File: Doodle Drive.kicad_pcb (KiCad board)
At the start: 2 copper layers, 62.9 x 80 mm, 101 parts, among them J1 USB_B, J12 PINHD_1x4_Male, J15 PINHD_1x4_Male, J2 PINHD_1x4_Male, J3 Screw_Terminal_01x02, J6 PINHD_1x2_Male, J8 PINHD_1x4_Male, J9 PINHD_1x4_Male, SW1 Push_Button, SW2 Push_Button, SW3 Push_Button, U1 STM32F411RETx, U2 DRV8825PWP, U3 DRV8825PWP, U4 DRV8825PWP, U5 DRV8825PWP, U6 AP7343-30W5-7, U7 CP2102-GMR_NRND, Y1 32.768KHz ±20ppm 12.5pF, Y2 25MHZ 9PF

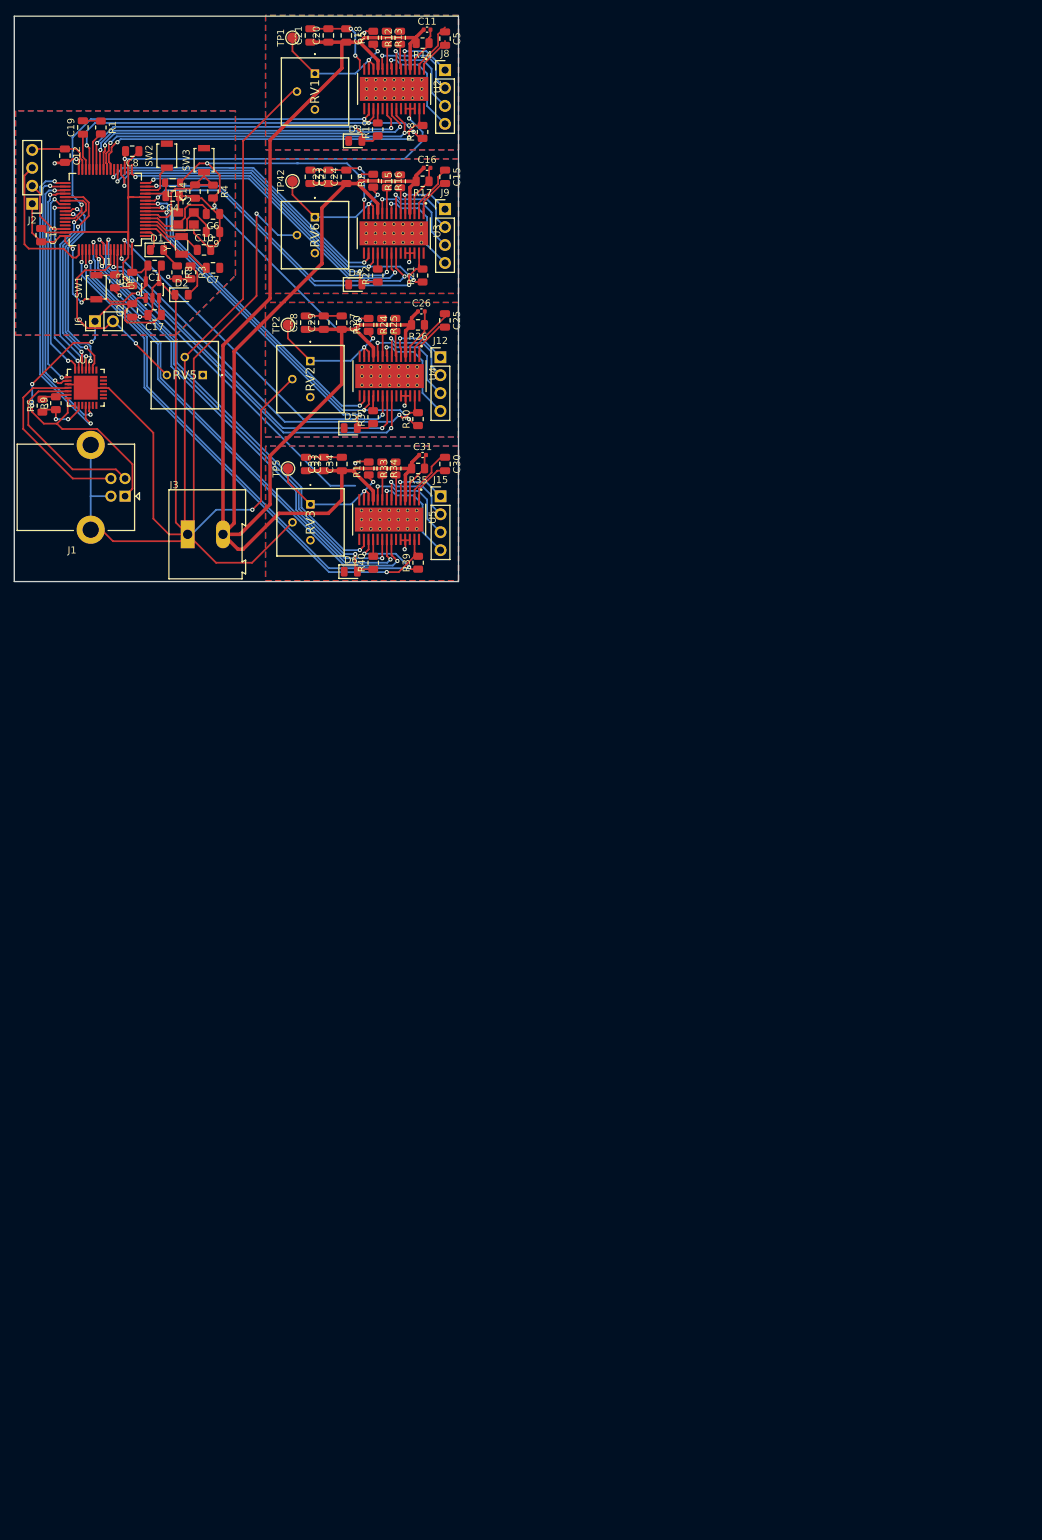
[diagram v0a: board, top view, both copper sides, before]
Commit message: deTommaso approved version
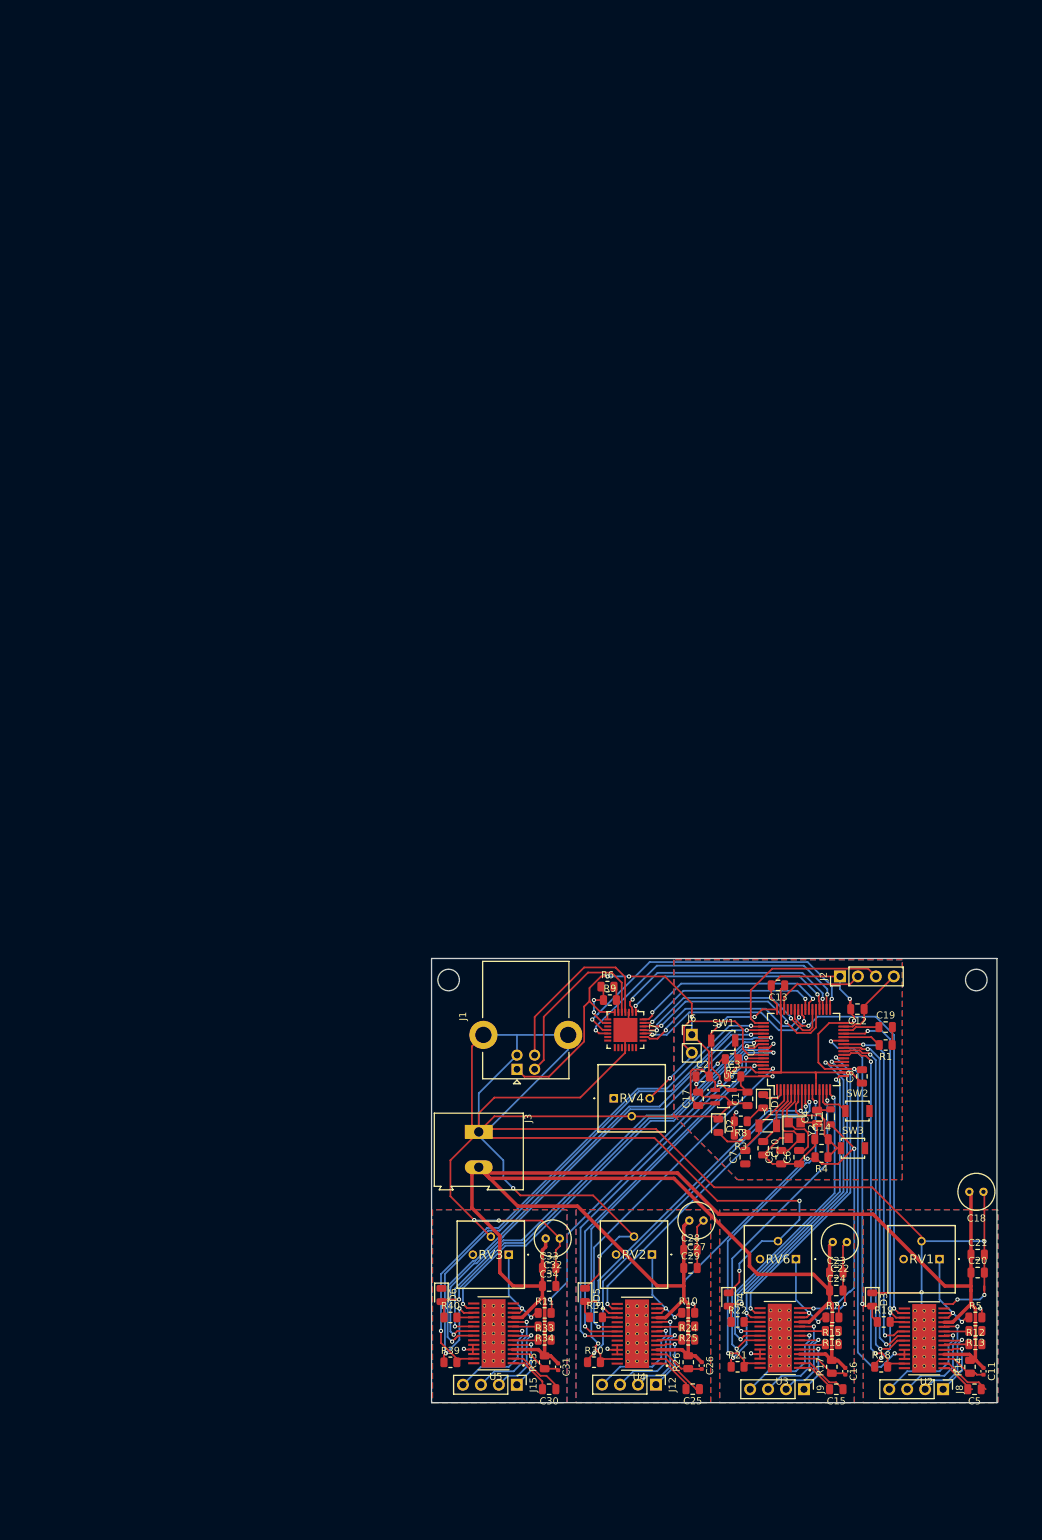
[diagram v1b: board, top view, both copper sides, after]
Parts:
- removed RV5: R_Potentiometer, poti:3386P1473LF
- removed TP1, TP2, TP42, TP5: TestPoint, TestPoint:TestPoint_Pad_D1.5mm
- added RV4: R_Potentiometer, poti:3386P1473LF, F.Cu at (84.8, 73.1)
- C18, C22, C27, C32: value Bulk Capacitance. 4.7uF? -> 10uF; footprint Capacitor_SMD:C_0805_2012Metric -> Capacitor_THT:C_Radial_D5.0mm_H5.0mm_P2.00mm
- moved C11 205.5 mm to (137.2, 111.8), turned to -90 degrees
- moved C5 205.3 mm to (135.9, 114.3), turned to 180 degrees
- moved R14 202.7 mm to (135.3, 111.1), turned to 90 degrees
- moved R12 202.0 mm to (136.0, 108.0), turned to 0 degrees
- moved R13 201.1 mm to (136.0, 106.0), turned to 180 degrees
- moved R5 200.1 mm to (136.0, 104.1), turned to 0 degrees
- moved J8 199.6 mm to (131.4, 114.3), turned to -90 degrees
- moved C20 197.7 mm to (136.3, 97.8), turned to 0 degrees
- moved C21 196.7 mm to (136.3, 95.2), turned to 0 degrees
- moved U2 192.1 mm to (128.8, 107.1), turned to 180 degrees
- moved RV1 189.6 mm to (130.9, 95.9), turned to 0 degrees
- moved C18 186.8 mm to (137.2, 86.4), turned to 180 degrees
- moved R18 186.4 mm to (122.7, 111.1), turned to 0 degrees
- moved R19 183.3 mm to (123.0, 104.8), turned to 0 degrees
- moved C16 180.3 mm to (117.6, 111.8), turned to -90 degrees
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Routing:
- net GND: track 407.9 -> 518.0 mm, vias 8 -> 14
- net +3V3: track 221.9 -> 241.3 mm
- net +15V: track 304.9 -> 320.9 mm
- net Net-(U2-AVREF): track 20.7 -> 14.3 mm
- net Net-(U5-AVREF): track 21.0 -> 14.6 mm
- net Net-(U3-AVREF): track 21.5 -> 15.1 mm
- net Net-(U4-AVREF): track 20.7 -> 14.4 mm
- net PA14: track 20.7 -> 25.5 mm
- net PA13: track 9.06 -> 13.4 mm
- net PB13: track 40.1 -> 43.0 mm
- net PB6: track 30.3 -> 28.2 mm
- net PB14: track 32.2 -> 34.2 mm
- net PB15: track 29.9 -> 31.6 mm
- net +5V: track 65.5 -> 67.1 mm
- net PB12: track 43.4 -> 44.8 mm
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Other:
- board size 62.9 x 80 mm -> 80 x 62.9 mm

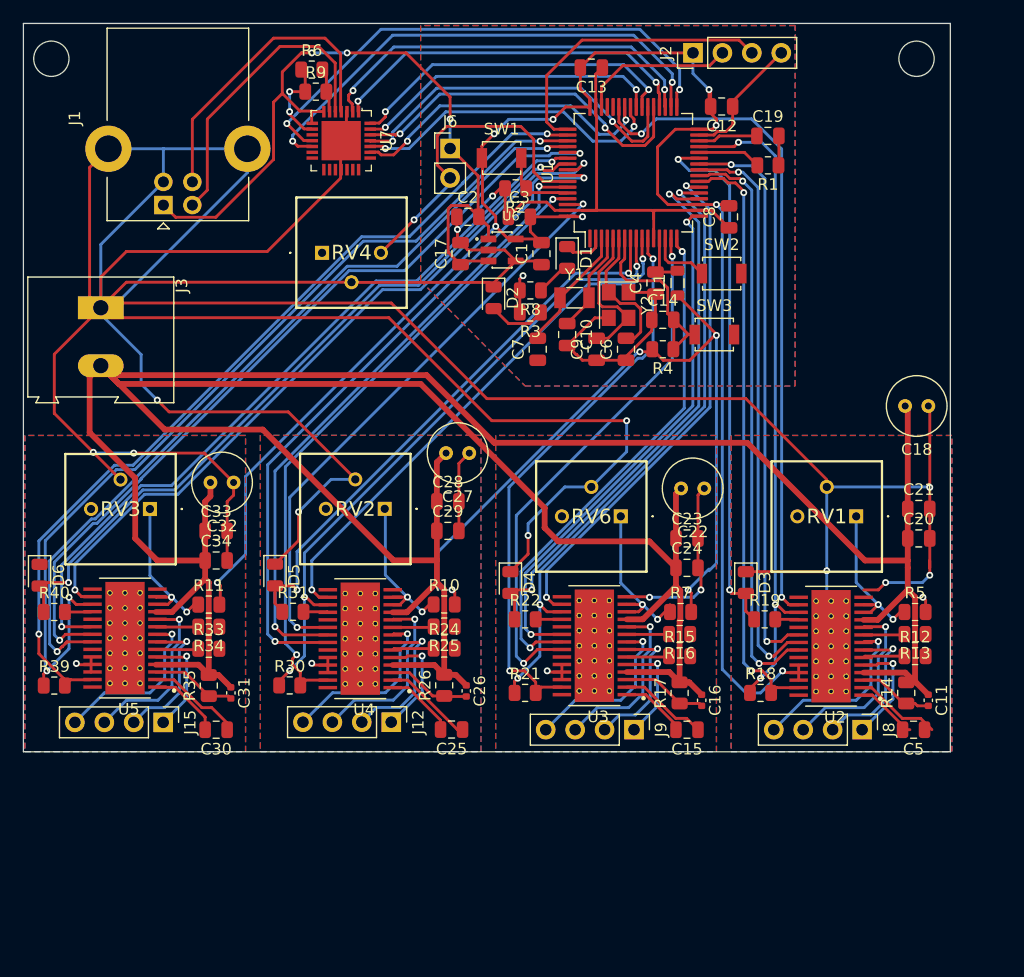
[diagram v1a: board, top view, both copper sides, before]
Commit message: bestellte version
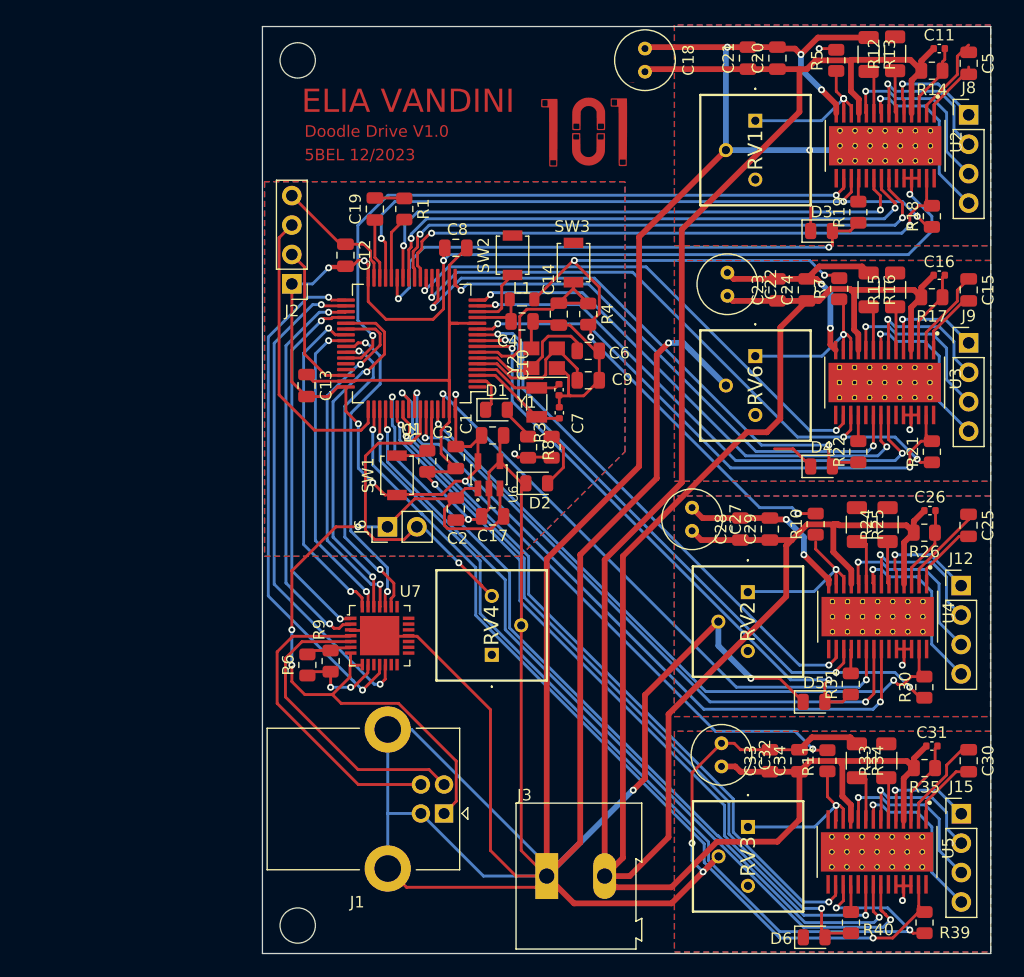
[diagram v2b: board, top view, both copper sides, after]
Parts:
- C10, C7: footprint Capacitor_SMD:C_0805_2012Metric -> Capacitor_SMD:C_0402_1005Metric
- C11, C16, C26, C31: value 100nF 16V ceramic -> 100nF
- C15, C25, C30, C5: value 10nF 50V -> 10nF
- C20, C21, C23, C24, C28, C29, C33, C34: value 100nF 50V -> 100nF
- C6, C9: value 12pF -> 18pF
- L1: value 10uH ±10% -> 10uH
- R12, R13, R15, R16, R24, R25, R33, R34: footprint Resistor_SMD:R_0805_2012Metric -> Resistor_SMD:R_1206_3216Metric
- R4: value 0 -> 0ohm
- U6: value AP7343-30W5-7 -> AP7343-33W5-7
- U7: value CP2102-GMR_NRND -> CP2102-GMR
- Y2: value 25MHZ 9PF -> 25MHZ 12PF
- moved R39 77.9 mm to (136.8, 130.9), turned to 90 degrees
- moved R40 73.8 mm to (130.5, 130.9), turned to 90 degrees
- moved D6 73.8 mm to (127.3, 132.2), turned to 0 degrees
- moved J15 69.3 mm to (140.0, 121.6), turned to 0 degrees
- moved U5 67.5 mm to (132.7, 124.8), turned to -90 degrees
- moved C30 65.0 mm to (140.6, 117.0), turned to -90 degrees
- moved J3 62.4 mm to (104.2, 126.9), turned to 0 degrees
- moved R35 62.2 mm to (136.8, 117.6), turned to 180 degrees
- moved C31 60.7 mm to (137.5, 115.7), turned to 0 degrees
- moved R33 59.3 mm to (133.5, 117.0), turned to 90 degrees
- moved RV3 58.5 mm to (121.6, 122.7), turned to 90 degrees
- moved J1 57.8 mm to (95.4, 121.5), turned to 180 degrees
- moved C5 57.7 mm to (140.6, 56.8), turned to -90 degrees
- moved R34 57.1 mm to (131.0, 117.0), turned to -90 degrees
- moved C11 56.3 mm to (138.1, 55.5), turned to 0 degrees
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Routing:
- net GND: track 518.0 -> 541.4 mm, vias 14 -> 15
- net +3V3: track 241.3 -> 235.8 mm
- net +15V: track 320.9 -> 325.6 mm
- net PC14: track 10.9 -> 8.61 mm
- net PC15: track 8.78 -> 7.83 mm
- net Net-(U3-AVREF): track 15.1 -> 14.9 mm, vias 2 -> 1
- net Net-(U5-AVREF): track 14.6 -> 14.8 mm, vias 2 -> 1
- net Net-(U4-AVREF): vias 2 -> 1
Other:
- board size 80 x 62.9 mm -> 62.9 x 80 mm
- board text added: "5BEL 12/2023"
- board text added: "Doodle Drive V1.0"
- board text added: "ELIA VANDINI"
